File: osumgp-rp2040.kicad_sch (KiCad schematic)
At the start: 76 parts, among them J1 USB_C_Receptacle_USB2.0, J2 SWD, J3 USB, J4 I2C, SW1 BOOTSEL, SW2 RST, SW3 Alpsalpine_RKJXV, SW4 Alpsalpine_RKJXV, U2 W25Q16JVUXIQ, U4 USBLC6-2P6, U5 RP2040, U8 AP2112K-3.3, Y1 ECS-120-12-36-AGN-TR3

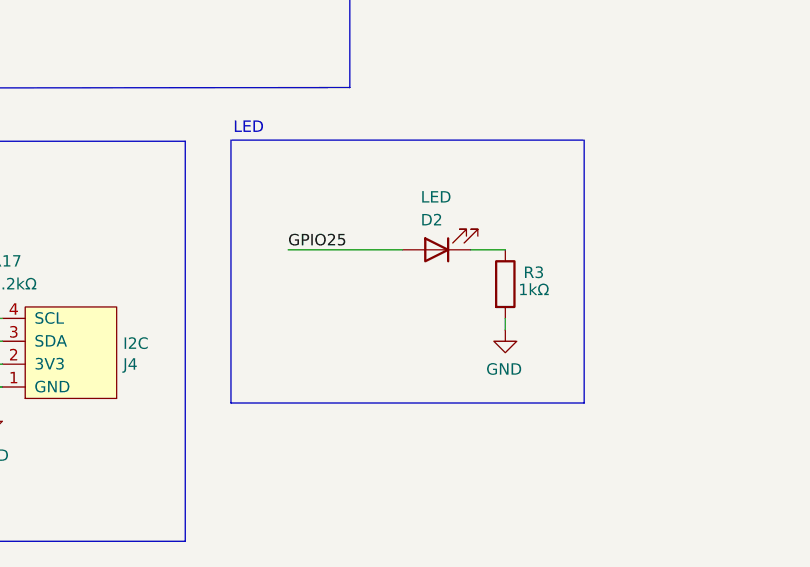
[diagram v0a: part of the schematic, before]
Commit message: fix led
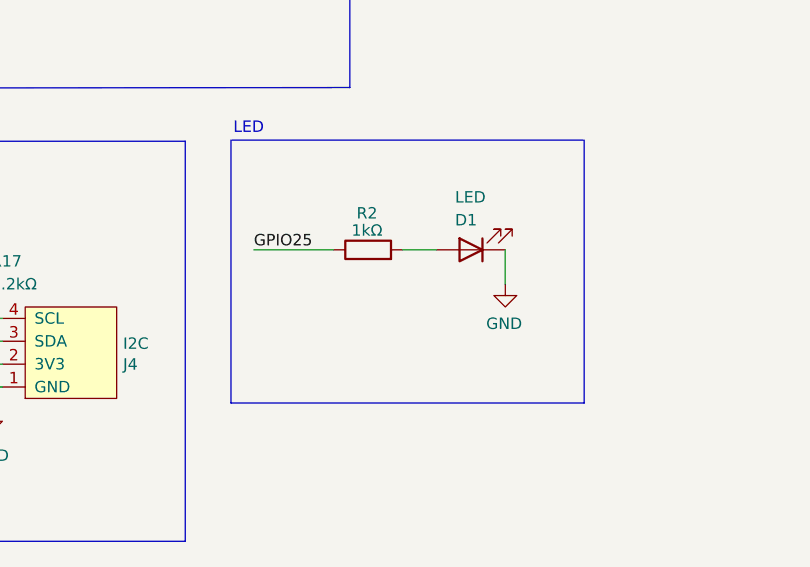
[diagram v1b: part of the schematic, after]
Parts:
- removed D2: LED, LED_SMD:LED_0603_1608Metric_Pad1.05x0.95mm_HandSolder, symbol Device:LED
- removed R3: 1kΩ, Resistor_SMD:R_0402_1005Metric, symbol Device:R
- added D1: LED, LED_SMD:LED_0603_1608Metric_Pad1.05x0.95mm_HandSolder, symbol Device:LED
- added R2: 1kΩ, Resistor_SMD:R_0402_1005Metric, symbol Device:R
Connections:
- net GND: now also D1.1 (K)
- net GPIO25: now also R2.1
- new net: D1.2 (A), R2.2
